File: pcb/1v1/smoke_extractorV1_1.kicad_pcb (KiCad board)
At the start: 2 copper layers, 54 x 27 mm, 48 parts, among them J1 USB_C_Receptacle, J2 Screw_Terminal_01x02, Q1 AO3400A, U1 LMV331, U2 RA11131100, U3 MP1542, U4 LMV331, U5 LMV331

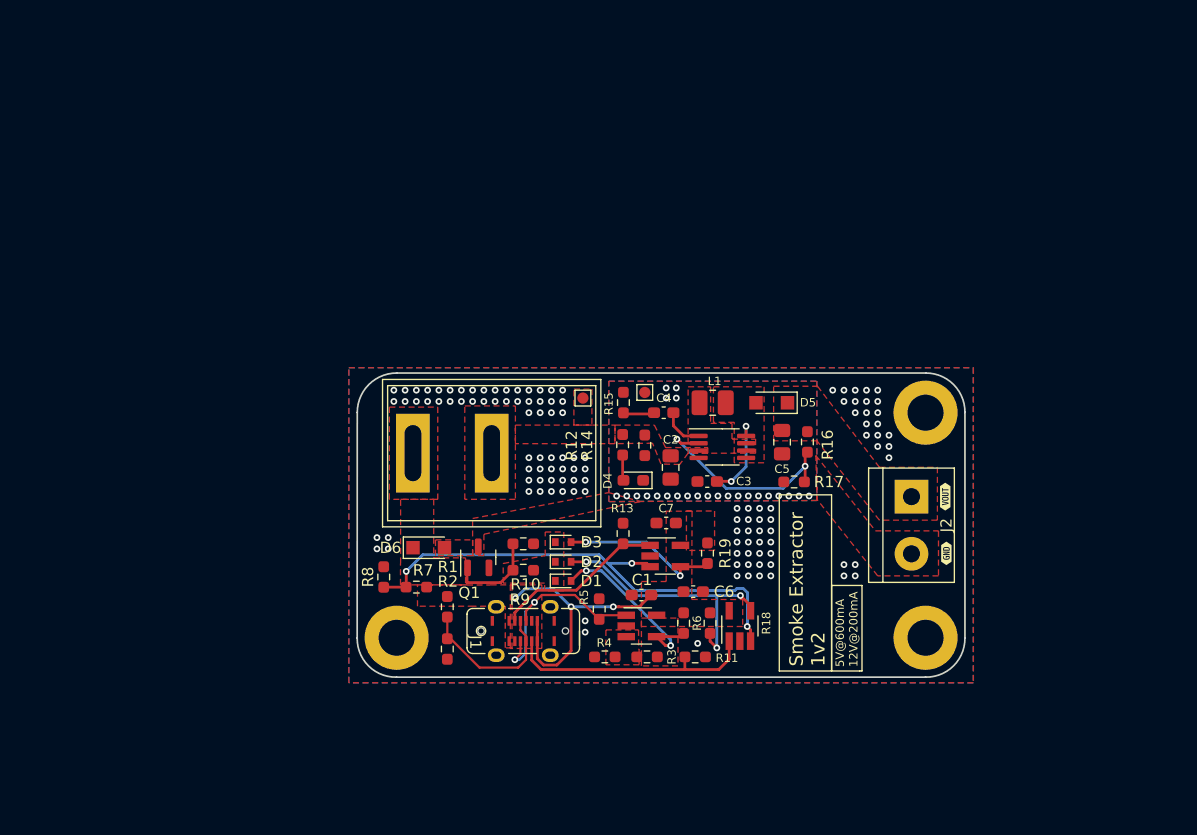
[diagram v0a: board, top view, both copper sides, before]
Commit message: smoke extractor 2.0
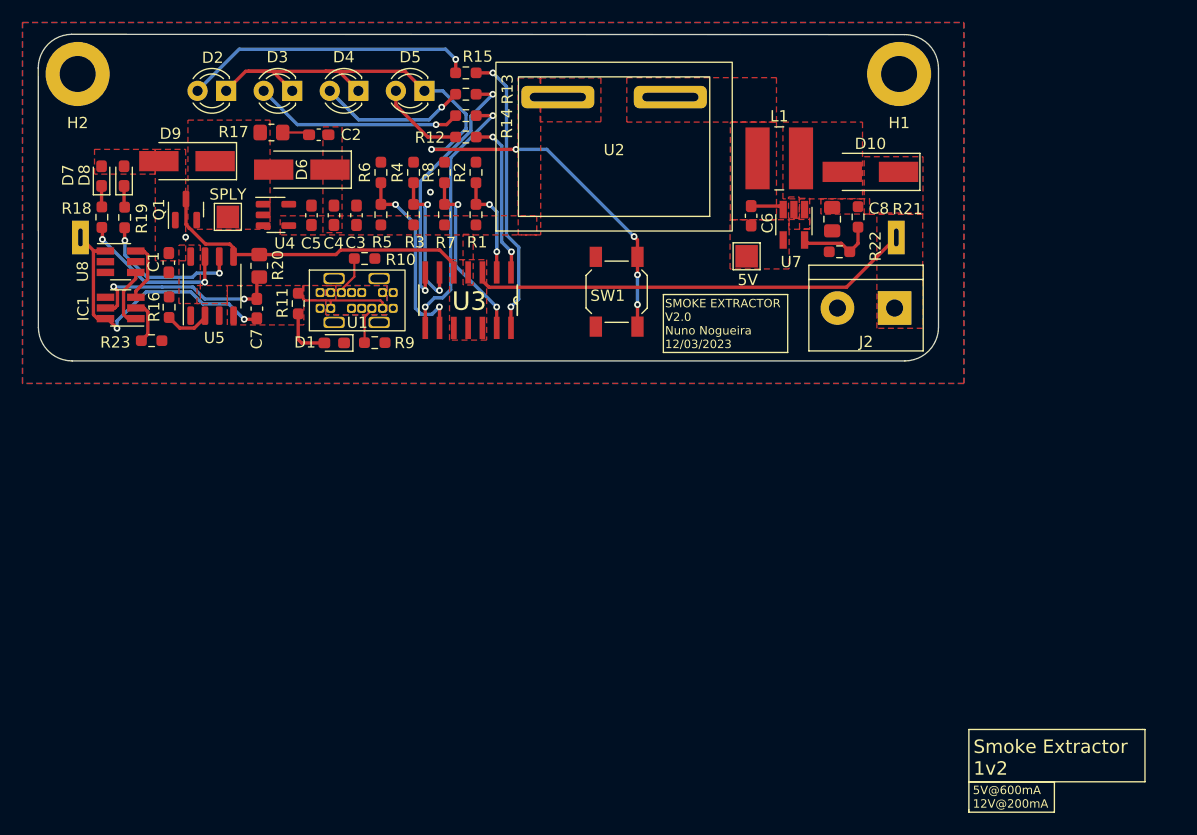
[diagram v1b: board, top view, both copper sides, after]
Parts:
- removed H3: MountingHole_Pad, MountingHole:MountingHole_3.2mm_M3_ISO7380_Pad
- removed J1: USB_C_Receptacle, CustomFootprints:USB4120-03-C
- removed REF** (x2): TestPoint_Pad_1.0x1.0mm, TestPoint:TestPoint_Pad_1.0x1.0mm
- removed kibuzzard-631C7DF6: G***, kibuzzard-631C7DF6
- removed kibuzzard-631C7E0D: G***, kibuzzard-631C7E0D
- added 5V: TestPoint, TestPoint:TestPoint_Pad_2.0x2.0mm, F.Cu at (126.8, 85.6)
- added C8: 22u, Capacitor_SMD:C_0805_2012Metric_Pad1.18x1.45mm_HandSolder, F.Cu at (134.4, 82.3)
- added D10: SS14, Diode_SMD:D_SMA_Handsoldering, F.Cu at (137.8, 78.1)
- added D7: RLED, LED_SMD:LED_0603_1608Metric_Pad1.05x0.95mm_HandSolder, F.Cu at (69.5, 78.5)
- added D8: GLED, LED_SMD:LED_0603_1608Metric_Pad1.05x0.95mm_HandSolder, F.Cu at (71.5, 78.5)
- added D9: SS14, Diode_SMD:D_SMA_Handsoldering, F.Cu at (77.1, 77.1)
- added IC1: DW01A, Package_TO_SOT_SMD:SOT-23-6_Handsoldering, F.Cu at (71.2, 90.2)
- added R20: 100, Resistor_SMD:R_0805_2012Metric_Pad1.20x1.40mm_HandSolder, F.Cu at (83.5, 86.4)
- added R21: 44.2k, Resistor_SMD:R_0603_1608Metric_Pad0.98x0.95mm_HandSolder, F.Cu at (136.8, 82.1)
- added R22: 5k1, Resistor_SMD:R_0603_1608Metric_Pad0.98x0.95mm_HandSolder, F.Cu at (135.1, 85.2)
- added R23: 1k, Resistor_SMD:R_0603_1608Metric_Pad0.98x0.95mm_HandSolder, F.Cu at (74.0, 93.1)
- added SPLY: TestPoint, TestPoint:TestPoint_Pad_2.0x2.0mm, F.Cu at (80.8, 82.1)
- added SW1: SW_Push, Button_Switch_SMD:SW_SPST_SKQG_WithStem, F.Cu at (115.3, 88.8)
- added U6: 18350-HOLDER, CustomFootprints:18350-Holder, B.Cu at (67.6, 83.9)
- added U7: ME2149FM5G, Package_TO_SOT_SMD:SOT-23-5_HandSoldering, F.Cu at (131.1, 82.8)
- added U8: FH8205, Package_TO_SOT_SMD:SOT-23-6_Handsoldering, F.Cu at (71.2, 86.1)
- C2: value 10u -> 120p; footprint Capacitor_SMD:C_0805_2012Metric_Pad1.18x1.45mm_HandSolder -> Capacitor_SMD:C_0603_1608Metric_Pad1.08x0.95mm_HandSolder
- C3: value 10n -> 10u
- C4: value 2.2n -> 10u
- C5: footprint Capacitor_SMD:C_0805_2012Metric_Pad1.18x1.45mm_HandSolder -> Capacitor_SMD:C_0603_1608Metric_Pad1.08x0.95mm_HandSolder
- C6: value 0.1u -> 10u
- D1: value D -> LED; footprint Diode_SMD:D_SOD-523 -> LED_SMD:LED_0603_1608Metric_Pad1.05x0.95mm_HandSolder
- D2, D3: value D -> 3mmWhite; footprint Diode_SMD:D_SOD-523 -> LED_THT:LED_D3.0mm
- D4: value LED -> 3mmWhite; footprint LED_SMD:LED_0603_1608Metric_Pad1.05x0.95mm_HandSolder -> LED_THT:LED_D3.0mm
- D5: value SS34 -> 3mmWhite; footprint Diode_SMD:Nexperia_CFP3_SOD-123W -> LED_THT:LED_D3.0mm
- D6: value SS34 -> SS14; footprint Diode_SMD:Nexperia_CFP3_SOD-123W -> Diode_SMD:D_SMA_Handsoldering
- L1: value 4.7u -> 3.3u; footprint Inductor_SMD:L_1008_2520Metric_Pad1.43x2.20mm_HandSolder -> Inductor_SMD:L_Wuerth_WE-PD2-Typ-MS
- Q1: value AO3400A -> FDN336P
- R1, R7: value 47k -> 3k6
- R11, R13: value 5.1k -> 1k
- R14: value 100k -> 1k
- R15: value 15k -> 1k
- R16: value 86.6k -> 1.2k
- R17: value 12k -> 5; footprint Resistor_SMD:R_0603_1608Metric_Pad0.98x0.95mm_HandSolder -> Resistor_SMD:R_0805_2012Metric_Pad1.20x1.40mm_HandSolder
- R18, R19: value 5k1 -> 1k
- R2: value 6k8 -> 16k
- R3, R5: value 47k -> 1k8
- R4: value 4k7 -> 5k1
- R6: value 5k1 -> 3k6
- R8: value 7k6 -> 5k1
- R9: value 100 -> 5k1
- U1: value LMV331 -> USB-TYPE-C-31-M-15; footprint Package_TO_SOT_SMD:SOT-23-5_HandSoldering -> CustomFootprints:USB-TYPE-C-31-M-15
- U2: value RA11131100 -> SDDJE; footprint CustomFootprints:RA11131100 -> CustomFootprints:SDDJE
- U3: value MP1542 -> LM324DT; footprint Package_SO:MSOP-8_3x3mm_P0.65mm -> Package_SO:SOIC127P600X175-14N
- U4: value LMV331 -> TPS613222ADBV; footprint Package_TO_SOT_SMD:SOT-23-5_HandSoldering -> Package_TO_SOT_SMD:SOT-23-5
- U5: value LMV331 -> TP4056; footprint Package_TO_SOT_SMD:SOT-23-5_HandSoldering -> Package_SO:SOP-8_3.9x4.9mm_P1.27mm
- moved H2 81.1 mm to (67.4, 69.4)
- moved H1 67.1 mm to (140.4, 69.4)
- moved R18 65.0 mm to (69.5, 82.1), turned to -90 degrees
- moved R19 59.8 mm to (71.6, 82.2), turned to -90 degrees
- moved R16 58.0 mm to (75.5, 90.1), turned to 90 degrees
- moved R17 55.9 mm to (84.6, 74.6), turned to 0 degrees
- moved U4 55.1 mm to (85.0, 81.9), turned to 0 degrees
- moved D2 51.5 mm to (80.6, 70.9), turned to 180 degrees
- moved C1 51.3 mm to (75.5, 86.2), turned to -90 degrees
- moved R6 48.2 mm to (94.3, 78.2)
- moved R11 47.2 mm to (87.0, 89.8), turned to -90 degrees
- moved U5 46.9 mm to (79.4, 88.2), turned to 90 degrees
- moved D3 46.8 mm to (86.5, 70.9), turned to 180 degrees
- moved C5 46.4 mm to (88.2, 82.0), turned to 90 degrees
- moved R4 46.3 mm to (97.2, 78.2), turned to 90 degrees
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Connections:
- C1 pad 1: VBUS_OPEN -> VBUS
- C1 pad 2: GND -> VBAT-PROTECT
- C2 pad 1: VBUS_SWITCH -> Net-(C2-Pad1)
- C2 pad 2: VBUS_DRAIN -> +5V
- C3 pad 1: Net-(C3-Pad1) -> +5V
- C3 pad 2: VBUS_DRAIN -> VBAT-PROTECT
- C4 pad 1: Net-(C4-Pad1) -> +5V
- C4 pad 2: Net-(C4-Pad2) -> VBAT-PROTECT
- C5 pad 1: VBOOST_OUT -> +5V
- C5 pad 2: VBUS_DRAIN -> VBAT-PROTECT
- C6 pad 1: VBUS_OPEN -> V5_SWITCH
- C6 pad 2: GND -> VBAT-PROTECT
- C7 pad 1: VBUS_OPEN -> Net-(C7-Pad1)
- C7 pad 2: GND -> Net-(C7-Pad2)
- D1 pad 1: Net-(D1-Pad1) -> VBAT-PROTECT
- D1 pad 2: CHG_DET -> Net-(D1-Pad2)
- D2 pad 1: Net-(D1-Pad1) -> Net-(D2-Pad1)
- D2 pad 2: CC1_DET -> Net-(D2-Pad2)
- D3 pad 1: Net-(D1-Pad1) -> Net-(D2-Pad1)
- D3 pad 2: CC2_DET -> Net-(D3-Pad2)
- D4 pad 1: VBUS_DRAIN -> Net-(D2-Pad1)
- D5 pad 1: VBOOST_OUT -> Net-(D2-Pad1)
- D6 pad 1: VBUS_OPEN -> +5V
- D6 pad 2: VBUS_DRAIN -> VSPLY
- H1 pad 1: GND -> VBAT-PROTECT
- H2 pad 1: GND -> VBAT-PROTECT
- J2 pad 1: VBOOST_OUT -> +12V
- J2 pad 2: VBUS_DRAIN -> VBAT-PROTECT
- L1 pad 1: VBUS_SWITCH -> V5_SWITCH
- L1 pad 2: Net-(D5-Pad2) -> Net-(D10-Pad2)
- Q1 pad 1: Net-(Q1-Pad1) -> VBUS
- Q1 pad 2: GND -> VSPLY
- Q1 pad 3: VBUS_DRAIN -> VBAT+PROTECT
- R1 pad 1: D+ -> +5V
- R1 pad 2: VBUS_OPEN -> Net-(R1-Pad2)
- R10 pad 1: Net-(Q1-Pad1) -> Net-(R10-Pad1)
- R10 pad 2: GND -> VBAT-PROTECT
- R11 pad 1: GND -> VBUS
- R11 pad 2: CC1 -> Net-(D1-Pad2)
- R12 pad 1: VBUS_SWITCH -> Net-(R12-Pad1)
- R12 pad 2: Net-(D4-Pad2) -> Net-(D5-Pad2)
- R13 pad 1: GND -> Net-(R13-Pad1)
- R13 pad 2: CC2 -> Net-(D4-Pad2)
- R14 pad 1: VBUS_SWITCH -> Net-(R14-Pad1)
- R14 pad 2: VBUS_DRAIN -> Net-(D3-Pad2)
- R15 pad 1: Net-(C4-Pad2) -> Net-(R15-Pad1)
- R15 pad 2: VBUS_DRAIN -> Net-(D2-Pad2)
- R16 pad 1: VBOOST_OUT -> Net-(R16-Pad1)
- R16 pad 2: Net-(R16-Pad2) -> VBAT-PROTECT
- R17 pad 1: Net-(R16-Pad2) -> VSPLY
- R17 pad 2: VBUS_DRAIN -> Net-(C2-Pad1)
- R18 pad 1: CC1_DET -> Net-(D7-Pad1)
- R18 pad 2: VBUS_OPEN -> Net-(R18-Pad2)
- R19 pad 1: CC2_DET -> Net-(D8-Pad1)
- R19 pad 2: VBUS_OPEN -> Net-(R19-Pad2)
- R2 pad 1: GND -> Net-(R1-Pad2)
- R2 pad 2: D+ -> VBAT-PROTECT
- R3 pad 1: VDAT_REF -> +5V
- R3 pad 2: VBUS_OPEN -> Net-(R3-Pad2)
- R4 pad 1: GND -> Net-(R3-Pad2)
- R4 pad 2: VDAT_REF -> VBAT-PROTECT
- R5 pad 1: D- -> +5V
- R5 pad 2: GND -> Net-(R5-Pad2)
- R6 pad 1: CHG_DET -> Net-(R5-Pad2)
- R6 pad 2: VBUS_OPEN -> VBAT-PROTECT
- R7 pad 1: V_CC_REF -> +5V
- R7 pad 2: VBUS_OPEN -> Net-(R7-Pad2)
- R8 pad 1: GND -> Net-(R7-Pad2)
- R8 pad 2: V_CC_REF -> VBAT-PROTECT
- R9 pad 1: Net-(Q1-Pad1) -> Net-(R9-Pad1)
- R9 pad 2: Net-(D1-Pad1) -> VBAT-PROTECT
- U1 pad 1: D- -> VBAT-PROTECT
- U1 pad 2: GND -> VBUS
- U1 pad 3: VDAT_REF -> Net-(R10-Pad1)
- U1 pad 4: CHG_DET -> Net-(R9-Pad1)
- U1 pad 5: VBUS_OPEN -> unconnected-(U1-Pad5)
- U2 pad 1: VBUS_OPEN -> +5V
- U2 pad 2: VBUS_SWITCH -> V5_SWITCH
- U3 pad 1: Net-(C4-Pad1) -> Net-(R12-Pad1)
- U3 pad 2: Net-(R16-Pad2) -> Net-(R1-Pad2)
- U3 pad 3: VBUS_SWITCH -> VBAT+PROTECT
- U3 pad 4: VBUS_DRAIN -> +5V
- U3 pad 5: Net-(D5-Pad2) -> VBAT+PROTECT
- U3 pad 6: VBUS_SWITCH -> Net-(R3-Pad2)
- U3 pad 7: VBUS_SWITCH -> Net-(R13-Pad1)
- U3 pad 8: Net-(C3-Pad1) -> Net-(R14-Pad1)
- U4 pad 1: CC1 -> VSPLY
- U4 pad 2: GND -> VBAT-PROTECT
- U4 pad 3: V_CC_REF -> unconnected-(U4-Pad3)
- U4 pad 4: CC1_DET -> +5V
- U4 pad 5: VBUS_OPEN -> unconnected-(U4-Pad5)
- U5 pad 1: CC2 -> VBAT-PROTECT
- U5 pad 2: GND -> Net-(R16-Pad1)
- U5 pad 3: V_CC_REF -> VBAT-PROTECT
- U5 pad 4: CC2_DET -> VBUS
- U5 pad 5: VBUS_OPEN -> VBAT+PROTECT
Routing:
- net VBAT+PROTECT: track 0.00 -> 68.8 mm
- net Net-(D2-Pad1): track 0.00 -> 66.3 mm, vias 0 -> 5
- net V_CC_REF: track 44.2 -> 0.00 mm, vias 3 -> 0
- net Net-(C7-Pad2): track 0.00 -> 26.9 mm, vias 0 -> 2
- net Net-(D2-Pad2): track 0.00 -> 26.1 mm, vias 0 -> 1
- net Net-(R15-Pad1): track 0.00 -> 25.4 mm, vias 0 -> 2
- net VBUS_OPEN: track 24.6 -> 0.00 mm, vias 3 -> 0
- net CC1_DET: track 24.2 -> 0.00 mm, vias 3 -> 0
- net Net-(R13-Pad1): track 0.00 -> 23.4 mm, vias 0 -> 2
- net Net-(R14-Pad1): track 0.00 -> 23.3 mm, vias 0 -> 2
- net CC1: track 22.5 -> 0.00 mm
- net Net-(R16-Pad2): track 18.7 -> 0.00 mm, vias 2 -> 0
- net Net-(D3-Pad2): track 0.00 -> 18.6 mm, vias 0 -> 1
- net D-: track 18.6 -> 0.00 mm, vias 2 -> 0
- net Net-(C7-Pad1): track 0.00 -> 18.2 mm, vias 0 -> 2
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- added copper zone on F.Cu, net +12V
- added copper zone on F.Cu, net +5V
- added copper zone on F.Cu, net Net-(D10-Pad2)
- added copper zone on F.Cu, net V5_SWITCH
- added copper zone on F.Cu, net VBAT+PROTECT
- added copper zone on B.Cu, net VBAT-PROTECT
- added copper zone on F.Cu, net VBAT-PROTECT
- added copper zone on B.Cu, net VBUS
- added copper zone on F.Cu, net VBUS
- added copper zone on F.Cu, net VSPLY
- removed copper zone on B.Cu, net GND
- removed copper zone on F.Cu, net GND
- removed copper zone on F.Cu, net Net-(D1-Pad1)
- removed copper zone on F.Cu, net Net-(D5-Pad2)
- removed copper zone on F.Cu, net VBOOST_OUT
- removed copper zone on B.Cu, net VBUS_DRAIN
- removed copper zone on F.Cu, net VBUS_DRAIN
- removed copper zone on F.Cu, net VBUS_OPEN
- removed copper zone on F.Cu, net VBUS_SWITCH
- removed copper zone on F.Cu, net VDAT_REF
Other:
- board size 54 x 27 mm -> 80 x 29 mm
- board text added: "SMOKE EXTRACTOR V2.0 Nuno Nogueira 12/03/2023"
